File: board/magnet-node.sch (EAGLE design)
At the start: 19 parts, among them X1 SMA-142-0701-801/806

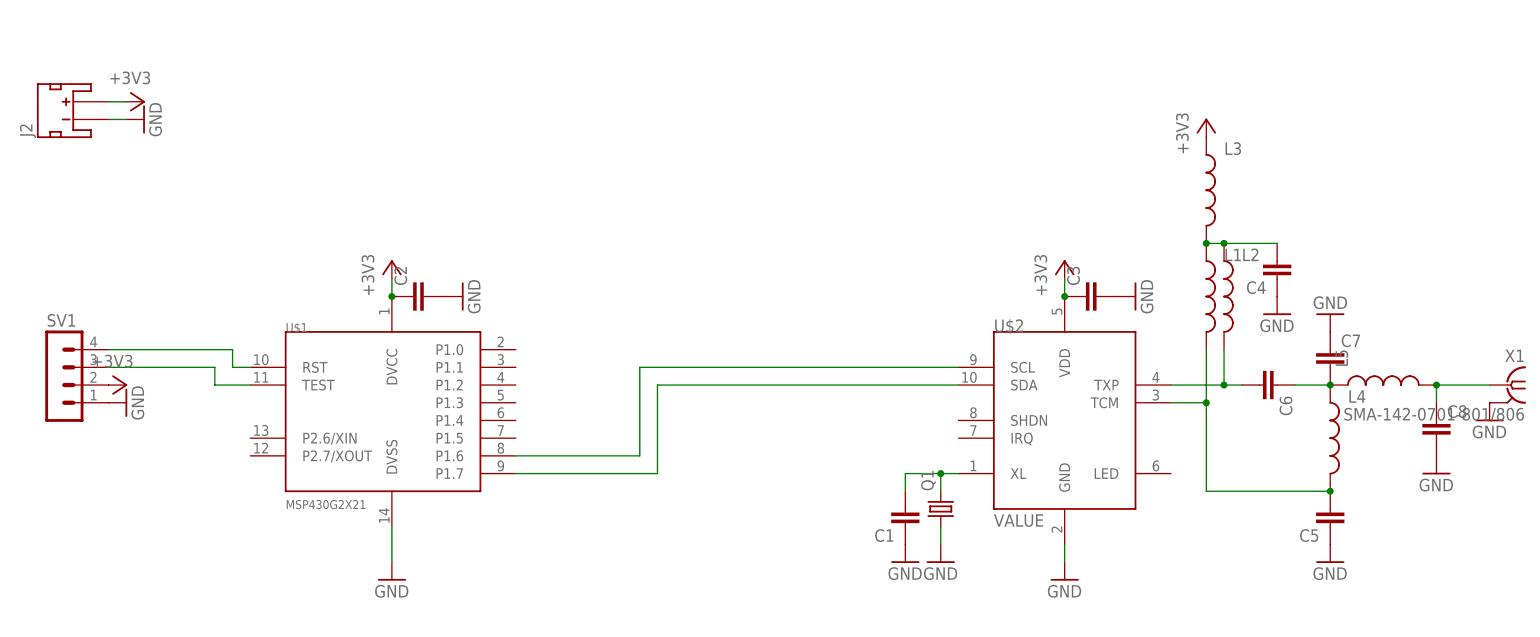
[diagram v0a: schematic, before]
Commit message: started pcb
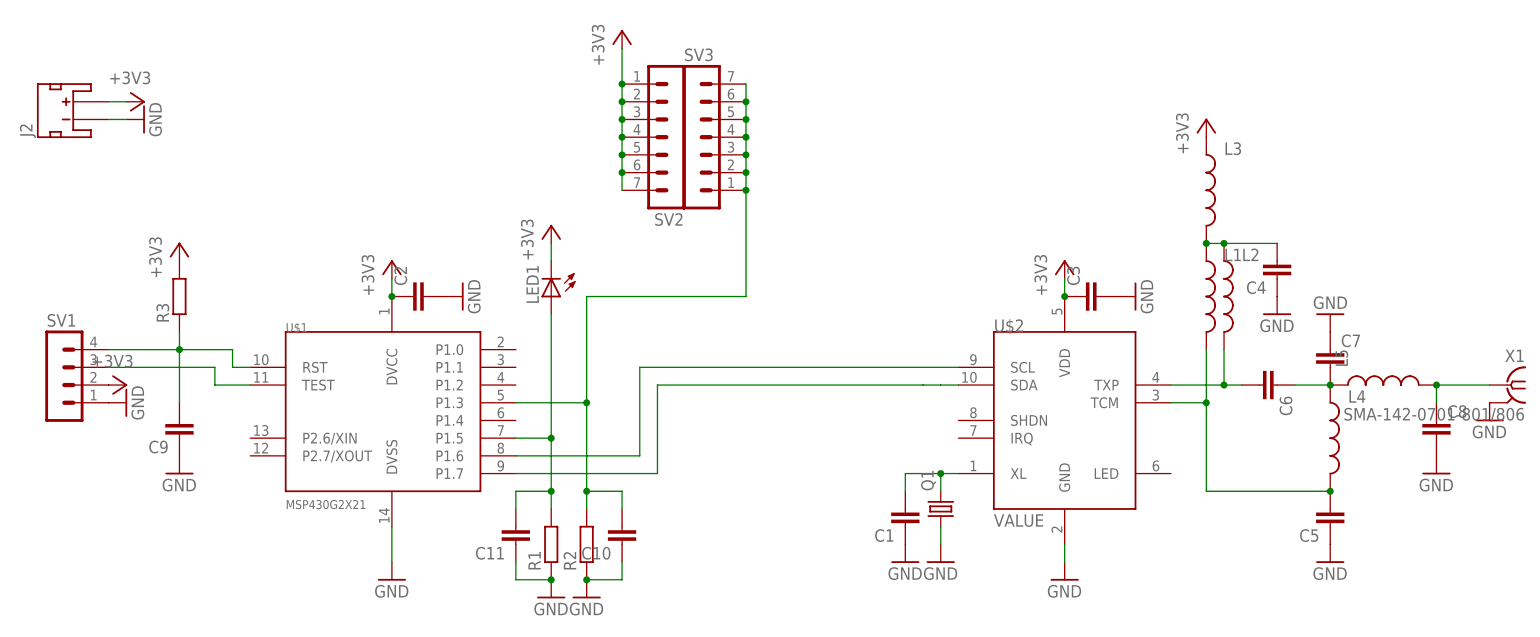
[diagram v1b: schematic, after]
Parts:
- added C10, C11, C9: (no value), rcl:C-EUC0603
- added LED1: (no value), led:LEDSMT1206
- added R1, R2, R3: (no value), rcl:R-EU_R0603
- added SV2, SV3: (no value), con-lstb:MA07-1
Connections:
- removed net N$1: SV1.4, U$1.RST
- new net N$12: C10.2, R2.2, SV3.1, SV3.2, SV3.3, SV3.4, SV3.5, SV3.6, SV3.7, U$1.P1.3
- new net N$13: C11.2, LED1.A, R1.2, U$1.P1.5
- new net N$15: C9.2, R3.1, SV1.4, U$1.RST
- net +3V3: now also LED1.C, R3.2, SV2.1, SV2.2, SV2.3, SV2.4, SV2.5, SV2.6, SV2.7
- net GND: now also C10.1, C11.1, C9.1, R1.1, R2.1
- net N$6: now also U$2.SDA
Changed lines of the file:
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@@
 <?xml version="1.0" encoding="utf-8"?>
 <!DOCTYPE eagle SYSTEM "eagle.dtd">
-<eagle version="7.1.0">
+<eagle version="6.5.0">
 <drawing>
 <settings>
@@
 <part name="X1" library="con-coax" deviceset="SMA-" device="142-0701-801/806"/>
 <part name="GND13" library="supply1" deviceset="GND" device=""/>
+<part name="SV2" library="con-lstb" deviceset="MA07-1" device=""/>
+<part name="SV3" library="con-lstb" deviceset="MA07-1" device=""/>
+<part name="R1" library="rcl" deviceset="R-EU_" device="R0603"/>
+<part name="R2" library="rcl" deviceset="R-EU_" device="R0603"/>
+<part name="LED1" library="led" deviceset="LED" device="SMT1206"/>
+<part name="+3V6" library="supply1" deviceset="+3V3" device=""/>
+<part name="GND14" library="supply1" deviceset="GND" device=""/>
+<part name="GND15" library="supply1" deviceset="GND" device=""/>
+<part name="+3V7" library="supply1" deviceset="+3V3" device=""/>
+<part name="R3" library="rcl" deviceset="R-EU_" device="R0603"/>
+<part name="C9" library="rcl" deviceset="C-EU" device="C0603"/>
+<part name="GND16" library="supply1" deviceset="GND" device=""/>
+<part name="+3V8" library="supply1" deviceset="+3V3" device=""/>
+<part name="C10" library="rcl" deviceset="C-EU" device="C0603"/>
+<part name="C11" library="rcl" deviceset="C-EU" device="C0603"/>
 </parts>
 <sheets>
@@
 <instance part="X1" gate="G1" x="205.74" y="45.72" rot="MR0"/>
 <instance part="GND13" gate="1" x="203.2" y="40.64"/>
+<instance part="SV2" gate="1" x="86.36" y="81.28" rot="R180"/>
+<instance part="SV3" gate="1" x="88.9" y="81.28"/>
+<instance part="R1" gate="G$1" x="68.58" y="22.86" rot="R90"/>
+<instance part="R2" gate="G$1" x="73.66" y="22.86" rot="R90"/>
+<instance part="LED1" gate="G$1" x="68.58" y="58.42" rot="R180"/>
+<instance part="+3V6" gate="G$1" x="68.58" y="68.58"/>
+<instance part="GND14" gate="1" x="73.66" y="15.24"/>
+<instance part="GND15" gate="1" x="68.58" y="15.24"/>
+<instance part="+3V7" gate="G$1" x="78.74" y="96.52"/>
+<instance part="R3" gate="G$1" x="15.24" y="58.42" rot="R90"/>
+<instance part="C9" gate="G$1" x="15.24" y="38.1" rot="R180"/>
+<instance part="GND16" gate="1" x="15.24" y="33.02"/>
+<instance part="+3V8" gate="G$1" x="15.24" y="66.04"/>
+<instance part="C10" gate="G$1" x="78.74" y="22.86" rot="R180"/>
+<instance part="C11" gate="G$1" x="63.5" y="22.86" rot="R180"/>
 </instances>
 <busses>
@@
 <pinref part="GND13" gate="1" pin="GND"/>
 </segment>
+<segment>
+<pinref part="R2" gate="G$1" pin="1"/>
+<pinref part="GND14" gate="1" pin="GND"/>
+<pinref part="C10" gate="G$1" pin="1"/>
+<wire x1="78.74" y1="20.32" x2="78.74" y2="17.78" width="0.1524" layer="91"/>
+<wire x1="78.74" y1="17.78" x2="73.66" y2="17.78" width="0.1524" layer="91"/>
+<junction x="73.66" y="17.78"/>
+</segment>
+<segment>
+<pinref part="R1" gate="G$1" pin="1"/>
+<pinref part="GND15" gate="1" pin="GND"/>
+<pinref part="C11" gate="G$1" pin="1"/>
+<wire x1="63.5" y1="20.32" x2="63.5" y2="17.78" width="0.1524" layer="91"/>
+<wire x1="63.5" y1="17.78" x2="68.58" y2="17.78" width="0.1524" layer="91"/>
+<junction x="68.58" y="17.78"/>
+</segment>
+<segment>
+<pinref part="C9" gate="G$1" pin="1"/>
+<pinref part="GND16" gate="1" pin="GND"/>
+</segment>
 </net>
 <net name="+3V3" class="0">
@@
 <pinref part="+3V5" gate="G$1" pin="+3V3"/>
 </segment>
-</net>
-<net name="N$1" class="0">
-<segment>
-<pinref part="U$1" gate="G$1" pin="RST"/>
-<wire x1="25.4" y1="48.26" x2="22.86" y2="48.26" width="0.1524" layer="91"/>
-<wire x1="22.86" y1="48.26" x2="22.86" y2="50.8" width="0.1524" layer="91"/>
-<wire x1="22.86" y1="50.8" x2="5.08" y2="50.8" width="0.1524" layer="91"/>
-<pinref part="SV1" gate="1" pin="4"/>
+<segment>
+<pinref part="+3V6" gate="G$1" pin="+3V3"/>
+<pinref part="LED1" gate="G$1" pin="C"/>
+<wire x1="68.58" y1="66.04" x2="68.58" y2="63.5" width="0.1524" layer="91"/>
+</segment>
+<segment>
+<pinref part="SV2" gate="1" pin="7"/>
+<wire x1="78.74" y1="73.66" x2="78.74" y2="76.2" width="0.1524" layer="91"/>
+<pinref part="SV2" gate="1" pin="6"/>
+<junction x="78.74" y="76.2"/>
+<wire x1="78.74" y1="76.2" x2="78.74" y2="78.74" width="0.1524" layer="91"/>
+<pinref part="SV2" gate="1" pin="5"/>
+<junction x="78.74" y="78.74"/>
+<wire x1="78.74" y1="78.74" x2="78.74" y2="81.28" width="0.1524" layer="91"/>
+<pinref part="SV2" gate="1" pin="4"/>
+<junction x="78.74" y="81.28"/>
+<wire x1="78.74" y1="81.28" x2="78.74" y2="83.82" width="0.1524" layer="91"/>
+<pinref part="SV2" gate="1" pin="3"/>
+<junction x="78.74" y="83.82"/>
+<wire x1="78.74" y1="83.82" x2="78.74" y2="86.36" width="0.1524" layer="91"/>
+<pinref part="SV2" gate="1" pin="2"/>
+<junction x="78.74" y="86.36"/>
+<wire x1="78.74" y1="86.36" x2="78.74" y2="88.9" width="0.1524" layer="91"/>
+<pinref part="SV2" gate="1" pin="1"/>
+<junction x="78.74" y="88.9"/>
+<wire x1="78.74" y1="88.9" x2="78.74" y2="93.98" width="0.1524" layer="91"/>
+<pinref part="+3V7" gate="G$1" pin="+3V3"/>
+</segment>
+<segment>
+<pinref part="R3" gate="G$1" pin="2"/>
+<pinref part="+3V8" gate="G$1" pin="+3V3"/>
 </segment>
 </net>
@@
 <net name="N$6" class="0">
 <segment>
-<wire x1="83.82" y1="45.72" x2="127" y2="45.72" width="0.1524" layer="91"/>
+<wire x1="83.82" y1="45.72" x2="121.92" y2="45.72" width="0.1524" layer="91"/>
+<wire x1="121.92" y1="45.72" x2="124.46" y2="45.72" width="0.1524" layer="91"/>
 <wire x1="83.82" y1="33.02" x2="83.82" y2="45.72" width="0.1524" layer="91"/>
 <pinref part="U$1" gate="G$1" pin="P1.7"/>
 <wire x1="63.5" y1="33.02" x2="83.82" y2="33.02" width="0.1524" layer="91"/>
+<pinref part="U$2" gate="G$1" pin="SDA"/>
+<wire x1="127" y1="45.72" x2="124.46" y2="45.72" width="0.1524" layer="91"/>
 </segment>
 </net>
@@
 </segment>
 </net>
+<net name="N$12" class="0">
+<segment>
+<pinref part="SV3" gate="1" pin="7"/>
+<wire x1="96.52" y1="88.9" x2="96.52" y2="86.36" width="0.1524" layer="91"/>
+<pinref part="SV3" gate="1" pin="6"/>
+<junction x="96.52" y="86.36"/>
+<wire x1="96.52" y1="86.36" x2="96.52" y2="83.82" width="0.1524" layer="91"/>
+<pinref part="SV3" gate="1" pin="5"/>
+<junction x="96.52" y="83.82"/>
+<wire x1="96.52" y1="83.82" x2="96.52" y2="81.28" width="0.1524" layer="91"/>
+<pinref part="SV3" gate="1" pin="4"/>
+<junction x="96.52" y="81.28"/>
+<wire x1="96.52" y1="81.28" x2="96.52" y2="78.74" width="0.1524" layer="91"/>
+<pinref part="SV3" gate="1" pin="3"/>
+<junction x="96.52" y="78.74"/>
+<wire x1="96.52" y1="78.74" x2="96.52" y2="76.2" width="0.1524" layer="91"/>
+<pinref part="SV3" gate="1" pin="2"/>
+<junction x="96.52" y="76.2"/>
+<wire x1="96.52" y1="76.2" x2="96.52" y2="73.66" width="0.1524" layer="91"/>
+<pinref part="SV3" gate="1" pin="1"/>
+<junction x="96.52" y="73.66"/>
+<pinref part="R2" gate="G$1" pin="2"/>
+<wire x1="73.66" y1="27.94" x2="73.66" y2="30.48" width="0.1524" layer="91"/>
+<wire x1="73.66" y1="30.48" x2="73.66" y2="43.18" width="0.1524" layer="91"/>
+<wire x1="73.66" y1="43.18" x2="73.66" y2="58.42" width="0.1524" layer="91"/>
+<wire x1="73.66" y1="58.42" x2="96.52" y2="58.42" width="0.1524" layer="91"/>
+<wire x1="96.52" y1="58.42" x2="96.52" y2="73.66" width="0.1524" layer="91"/>
+<pinref part="U$1" gate="G$1" pin="P1.3"/>
+<wire x1="63.5" y1="43.18" x2="73.66" y2="43.18" width="0.1524" layer="91"/>
+<junction x="73.66" y="43.18"/>
+<pinref part="C10" gate="G$1" pin="2"/>
+<wire x1="78.74" y1="27.94" x2="78.74" y2="30.48" width="0.1524" layer="91"/>
+<wire x1="78.74" y1="30.48" x2="73.66" y2="30.48" width="0.1524" layer="91"/>
+<junction x="73.66" y="30.48"/>
+</segment>
+</net>
+<net name="N$13" class="0">
+<segment>
+<pinref part="LED1" gate="G$1" pin="A"/>
+<pinref part="R1" gate="G$1" pin="2"/>
+<wire x1="68.58" y1="55.88" x2="68.58" y2="38.1" width="0.1524" layer="91"/>
+<wire x1="68.58" y1="38.1" x2="68.58" y2="30.48" width="0.1524" layer="91"/>
+<wire x1="68.58" y1="30.48" x2="68.58" y2="27.94" width="0.1524" layer="91"/>
+<pinref part="C11" gate="G$1" pin="2"/>
+<wire x1="63.5" y1="27.94" x2="63.5" y2="30.48" width="0.1524" layer="91"/>
+<wire x1="63.5" y1="30.48" x2="68.58" y2="30.48" width="0.1524" layer="91"/>
+<junction x="68.58" y="30.48"/>
+<pinref part="U$1" gate="G$1" pin="P1.5"/>
+<wire x1="63.5" y1="38.1" x2="68.58" y2="38.1" width="0.1524" layer="91"/>
+<junction x="68.58" y="38.1"/>
+</segment>
+</net>
+<net name="N$15" class="0">
+<segment>
+<pinref part="C9" gate="G$1" pin="2"/>
+<pinref part="R3" gate="G$1" pin="1"/>
+<wire x1="15.24" y1="43.18" x2="15.24" y2="50.8" width="0.1524" layer="91"/>
+<pinref part="U$1" gate="G$1" pin="RST"/>
+<wire x1="25.4" y1="48.26" x2="22.86" y2="48.26" width="0.1524" layer="91"/>
+<wire x1="22.86" y1="48.26" x2="22.86" y2="50.8" width="0.1524" layer="91"/>
+<wire x1="22.86" y1="50.8" x2="15.24" y2="50.8" width="0.1524" layer="91"/>
+<pinref part="SV1" gate="1" pin="4"/>
+<wire x1="15.24" y1="50.8" x2="5.08" y2="50.8" width="0.1524" layer="91"/>
+<wire x1="15.24" y1="53.34" x2="15.24" y2="50.8" width="0.1524" layer="91"/>
+<junction x="15.24" y="50.8"/>
+</segment>
+</net>
